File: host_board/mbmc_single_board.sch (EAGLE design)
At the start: 118 parts, among them IC1 ULN2803, IC15 PIC18F57K42-E_PT, IC16 REF3440IDBVR, IC17 MAX232, IC2 DIP Socket, IC3 REF02 5 VOLTS, IC4 5 VOLTS, IC5 12 VOLTS, IC6 3.3 VOLTS, J1 1-1586043-4, J2 1586044-4, Q3 ASF1, X15 RX-2, X16 TX-2, X17 RESETJMP

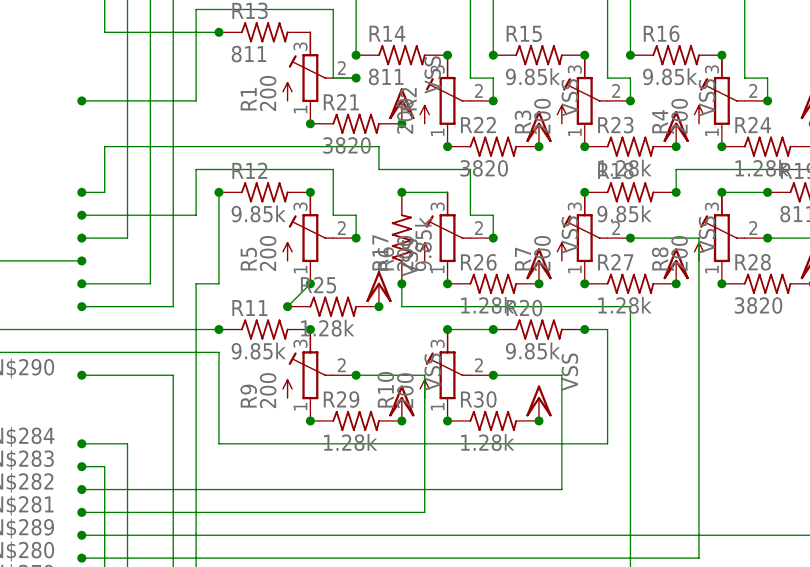
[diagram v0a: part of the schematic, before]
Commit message: up
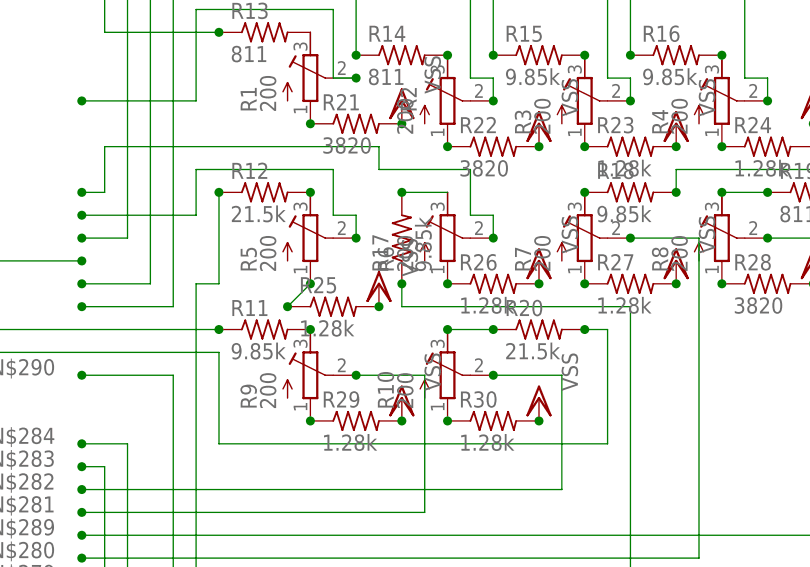
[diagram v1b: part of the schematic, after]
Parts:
- R12, R20: value 9.85k -> 21.5k
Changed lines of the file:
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@@
 <part name="R10" library="rcl" library_urn="urn:adsk.eagle:library:334" deviceset="R-TRIMM" device="3339P" package3d_urn="urn:adsk.eagle:package:23757/1" value="200"/>
 <part name="R11" library="rcl" library_urn="urn:adsk.eagle:library:334" deviceset="R-US_" device="R0805" package3d_urn="urn:adsk.eagle:package:23553/2" value="9.85k"/>
-<part name="R12" library="rcl" library_urn="urn:adsk.eagle:library:334" deviceset="R-US_" device="R0805" package3d_urn="urn:adsk.eagle:package:23553/2" value="9.85k"/>
+<part name="R12" library="rcl" library_urn="urn:adsk.eagle:library:334" deviceset="R-US_" device="R0805" package3d_urn="urn:adsk.eagle:package:23553/2" value="21.5k"/>
 <part name="R13" library="rcl" library_urn="urn:adsk.eagle:library:334" deviceset="R-US_" device="R0805" package3d_urn="urn:adsk.eagle:package:23553/2" value="811"/>
 <part name="R14" library="rcl" library_urn="urn:adsk.eagle:library:334" deviceset="R-US_" device="R0805" package3d_urn="urn:adsk.eagle:package:23553/2" value="811"/>
@@
 <part name="R18" library="rcl" library_urn="urn:adsk.eagle:library:334" deviceset="R-US_" device="R0805" package3d_urn="urn:adsk.eagle:package:23553/2" value="9.85k"/>
 <part name="R19" library="rcl" library_urn="urn:adsk.eagle:library:334" deviceset="R-US_" device="R0805" package3d_urn="urn:adsk.eagle:package:23553/2" value="811"/>
-<part name="R20" library="rcl" library_urn="urn:adsk.eagle:library:334" deviceset="R-US_" device="R0805" package3d_urn="urn:adsk.eagle:package:23553/2" value="9.85k"/>
+<part name="R20" library="rcl" library_urn="urn:adsk.eagle:library:334" deviceset="R-US_" device="R0805" package3d_urn="urn:adsk.eagle:package:23553/2" value="21.5k"/>
 <part name="R21" library="rcl" library_urn="urn:adsk.eagle:library:334" deviceset="R-US_" device="R0805" package3d_urn="urn:adsk.eagle:package:23553/2" value="3820"/>
 <part name="R22" library="rcl" library_urn="urn:adsk.eagle:library:334" deviceset="R-US_" device="R0805" package3d_urn="urn:adsk.eagle:package:23553/2" value="3820"/>
